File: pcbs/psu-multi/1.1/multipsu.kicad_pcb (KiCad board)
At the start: 2 copper layers, 85 x 55 mm, 56 parts, among them J1 Conn_01x06_Pin, J2 Conn_01x03_Male, J3 Conn_01x02_Pin, J4 Conn_01x03_Pin, J5 Conn_01x03_Pin, J6 Conn_01x02_Pin, J7 Conn_01x03_Pin, U1 LM337_SOT223, U2 LM317_SOT-223, U3 ZLDO1117QG33TA, U4 AMS1117-5.0, U5 NCP1117-12, U6 TMP100, U7 AP64351SP-13

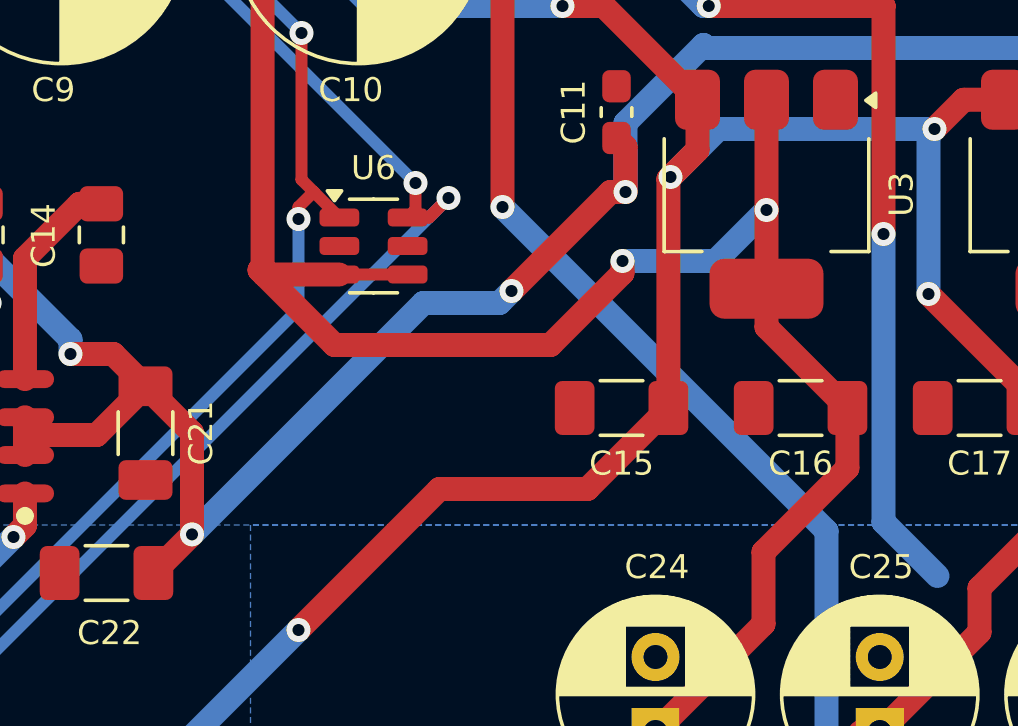
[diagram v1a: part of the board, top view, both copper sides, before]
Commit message: Updates
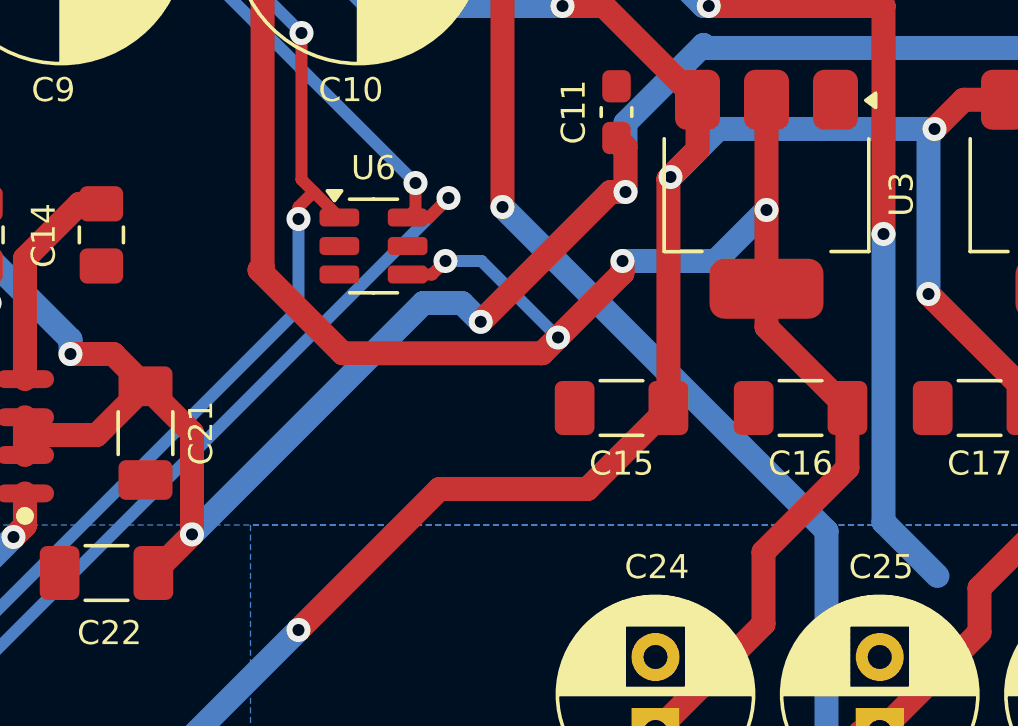
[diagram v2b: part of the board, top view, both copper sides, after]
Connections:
- U6 pad 3: 3V3 -> PGND
- U6 pad 5: PGND -> unconnected-(U6-ADD0-Pad5)
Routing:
- net 3V3: track 86.3 -> 88.0 mm, vias 2 -> 4
- net VP: track 134.7 -> 135.3 mm
